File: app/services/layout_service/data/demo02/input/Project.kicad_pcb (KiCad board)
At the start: 2 copper layers, 48 x 48 mm, 57 parts, among them J1 M50-3500542, J2 NATTREY, T1 Thermistor_NTC, U1 AP7366-W5-7, U2 DRDC3105F-7, U3 TCM809RVNB713, U4 ATSAMD21G18A-MUT, U5 MX25L4006EM2I-12G, U6 LM35DZ/NOPB, U7 VEML6040A3OG, U8 ISM330DHCXTR, U9 BQ25101YFPR, X1 12 MHz, X2 32.768 kHz

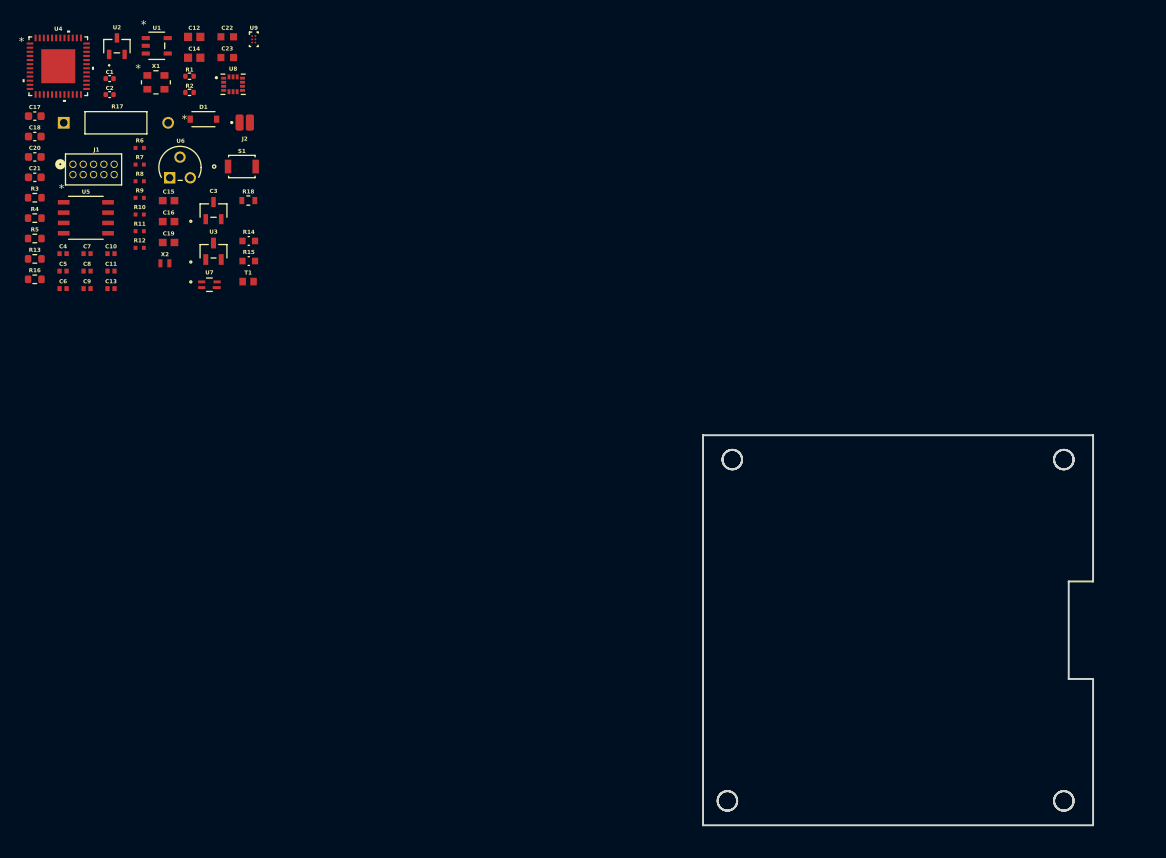
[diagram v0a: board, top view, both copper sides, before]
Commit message: 流程适配-反写网表-v2
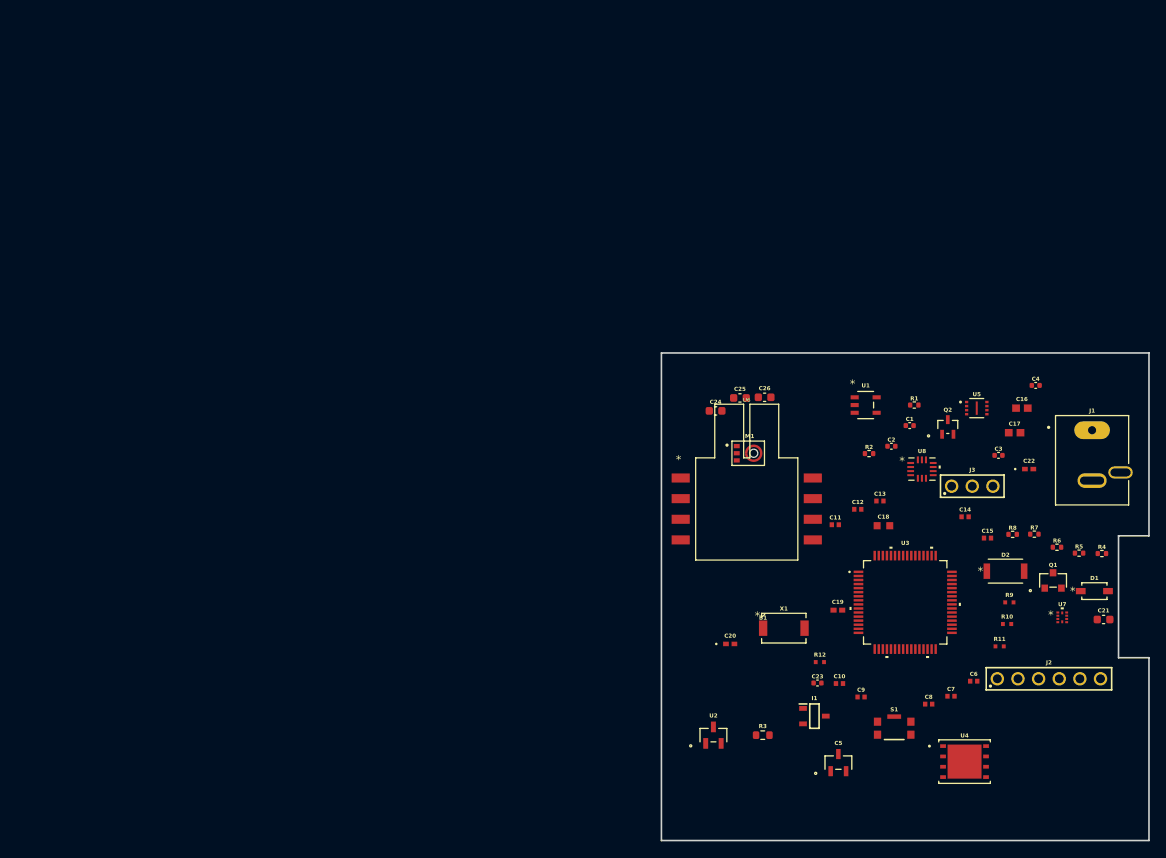
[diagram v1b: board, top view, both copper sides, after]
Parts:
- removed R13: 75R, LM35DZNOPB:R_0603_1608Metric
- removed R14, R15: 2.2K, VEML6040A3OG:RC0603N_YAG
- removed R16: 10k, ISM330DHCXTR:R_0603_1608Metric
- removed R17: 6K, BQ25101YFPR:CMF55_VIS
- removed R18: 1.35K, BQ25101YFPR:RES_RN73R_1J_KOA
- removed T1: Thermistor_NTC, BQ25101YFPR:TRES_NCP18XH103F03RB_MUR
- removed U9: BQ25101YFPR, BQ25101YFPR:YFP0006AFAV
- removed X2: 32.768 kHz, ATSAMD21G18A-MUT:ABS05_32_768KHZ_T
- added B1: Battery_CR1225, Battery_CR1225, F.Cu at (137.5, 109.2)
- added C24: C_0603_1608Metric, C_0603_1608Metric, F.Cu at (131.7, 77.1)
- added C25: C_0603_1608Metric, C_0603_1608Metric, F.Cu at (134.7, 75.5)
- added C26: C_0603_1608Metric, C_0603_1608Metric, F.Cu at (137.7, 75.5)
- added D2: SDO_CFP5_SOD128_NEX, SDO_CFP5_SOD128_NEX, F.Cu at (167.3, 96.8)
- added I1: SOT95P285X113-3N, SOT95P285X113-3N, F.Cu at (143.8, 114.7)
- added J3: 61300311121, 61300311121, F.Cu at (163.3, 86.4)
- added M1: MIC_ICS-40720, MIC_ICS-40720, F.Cu at (136.4, 82.3)
- added Q1: SOT-23_DIO, SOT-23_DIO, F.Cu at (173.2, 98.0)
- added Q2: SOT-323_DIO, SOT-323_DIO, F.Cu at (160.2, 79.1)
- C1, C2: value 1uF -> C_0402_1005Metric; footprint AP7366_W5_7:C_0402_1005Metric -> C_0402_1005Metric
- C10: value 1uF -> CAPC1005X55N; footprint ATSAMD21G18A-MUT:0402C -> 0402C
- C11, C6, C7: value 0.1uF -> CAPC1005X55N; footprint ATSAMD21G18A-MUT:0402C -> 0402C
- C12, C14: value 10uF -> CAPC1005X55N; footprint ATSAMD21G18A-MUT:0603C -> 0402C
- C13, C8: value 12 pF -> CAPC1005X55N; footprint ATSAMD21G18A-MUT:0402C -> 0402C
- C15: value 0.1uF -> CAPC1005X55N; footprint MX25L4006EM2I-12G:YAG_CC0603_YAG -> 0402C
- C16: value 0.01uF -> YAG_CC0603_YAG; footprint MX25L4006EM2I-12G:YAG_CC0603_YAG -> YAG_CC0603_YAG
- C17: value 0.01uF -> YAG_CC0603_YAG; footprint LM35DZNOPB:C_0603_1608Metric -> YAG_CC0603_YAG
- C18: value 1uF -> CAP_CL10A105KB8NNN_SAM; footprint LM35DZNOPB:C_0603_1608Metric -> CAP_CL10A105KB8NNN_SAM
- C19: value 0.1uF -> 0402_AVX; footprint VEML6040A3OG:YAG_CC0603_YAG -> 0402_AVX
- C20: value 0.1 uF -> CAP_0402_SAM; footprint ISM330DHCXTR:C_0603_1608Metric -> CAP_0402_SAM
- C21: value 0.1 uF -> C_0603_1608Metric; footprint ISM330DHCXTR:C_0603_1608Metric -> C_0603_1608Metric
- C22: value 1uF -> CAP_0402_SAM; footprint BQ25101YFPR:CAP_CL10A105KB8NNN_SAM -> CAP_0402_SAM
- C23: value 1uF -> C_0402_1005Metric; footprint BQ25101YFPR:CAP_CL10A105KB8NNN_SAM -> C_0402_1005Metric
- C3: value SM712-02HTG -> C_0402_1005Metric; footprint SM712-02HTG:SOT23-3_LTF -> C_0402_1005Metric
- C4: value 10 pF -> C_0402_1005Metric; footprint ATSAMD21G18A-MUT:0402C -> C_0402_1005Metric
- C5: value 0.1uF -> SOT23-3_LTF; footprint ATSAMD21G18A-MUT:0402C -> SOT23-3_LTF
- C9: value 10 pF -> CAPC1005X55N; footprint ATSAMD21G18A-MUT:0402C -> 0402C
- D1: value KDZVTR6.2B -> SOD-123_ONS; footprint DRDC3105F:DIO_KDZLVTF100_ROM -> SOD-123_ONS
- J1: value M50-3500542 -> CUI_PJ-044A; footprint ATSAMD21G18A-MUT:M50_3500542 -> CUI_PJ-044A
- J2: value NATTREY -> 61300611121; footprint BQ25101YFPR:SolderWirePad_1x02_SMD_1x2mm -> 61300611121
- R1: value 210K -> R_0402_1005Metric; footprint AP7366_W5_7:R_0402_1005Metric -> R_0402_1005Metric
- R10: value 1k -> RES_ERJ-2GEJ103X; footprint ATSAMD21G18A-MUT:0402R -> 0402R
- R11: value 330 -> RES_ERJ-2GEJ103X; footprint ATSAMD21G18A-MUT:0402R -> 0402R
- R12: value 10k -> RES_ERJ-2GEJ103X; footprint ATSAMD21G18A-MUT:0402R -> 0402R
- R2: value 40K -> R_0402_1005Metric; footprint AP7366_W5_7:R_0402_1005Metric -> R_0402_1005Metric
- R3: value 33K -> R_0603_1608Metric; footprint DRDC3105F:R_0603_1608Metric -> R_0603_1608Metric
- R4: value 1K -> R_0402_1005Metric; footprint DRDC3105F:R_0603_1608Metric -> R_0402_1005Metric
- R5: value 100K -> R_0402_1005Metric; footprint TCM809:R_0603_1608Metric -> R_0402_1005Metric
- R6, R7, R8: value 4.7k -> R_0402_1005Metric; footprint ATSAMD21G18A-MUT:0402R -> R_0402_1005Metric
- R9: value 4.7k -> RES_ERJ-2GEJ103X; footprint ATSAMD21G18A-MUT:0402R -> 0402R
- S1: value B3U-1000P -> SW_KMR221GLFS; footprint ATSAMD21G18A-MUT:B3U-1000P -> KMR221GLFS
- U1: value AP7366-W5-7 -> SOT25_DIO; footprint AP7366_W5_7:SOT25_DIO -> SOT25_DIO
- U2: value DRDC3105F-7 -> SOT-23_MC_MCH; footprint DRDC3105F:SOT23_MMBT2222A_NEX -> SOT-23_MC_MCH
- U3: value TCM809RVNB713 -> LQFP64-10x10mm; footprint TCM809:SOT-23_MC_MCH -> STM32F103RET6
- U4: value ATSAMD21G18A-MUT -> MR25H40CDC_EVS; footprint ATSAMD21G18A-MUT:QFN48_7X7MC_MCH -> MR25H40CDC_EVS
- U5: value MX25L4006EM2I-12G -> 8L_USON_2X3_ISI; footprint MX25L4006EM2I-12G:SOIC8_SOP8L_MAC -> 8L_USON_2X3_ISI
- U6: value LM35DZ/NOPB -> 1351-01_NXP; footprint LM35DZNOPB:Z03A -> 1351-01_NXP
- U7: value VEML6040A3OG -> MC3635_MEM; footprint VEML6040A3OG:LED_VEML6040A3OG_VIS -> MC3635_MEM
- U8: value ISM330DHCXTR -> BMX160_BOS; footprint ISM330DHCXTR:PQFN50P250X300X86-14N -> BMX160_BOS
- X1: value 12 MHz -> XTAL_NX5032GA-16.000M-STD-CSU-2_NDK; footprint ATSAMD21G18A-MUT:ABM8G_12_000MHZ_B4Y_T -> NX5032GA_16_000M_STD_CSU_2
- moved C21 142.3 mm to (179.4, 102.8)
- moved U4 140.6 mm to (162.3, 120.3)
- moved R4 137.7 mm to (179.2, 94.7)
- moved R5 134.2 mm to (176.4, 94.6)
- moved J1 130.6 mm to (178.0, 83.2)
- moved C17 126.7 mm to (168.5, 79.8)
- moved D1 124.1 mm to (178.3, 99.3)
- moved R6 123.1 mm to (173.7, 93.9)
- moved C6 122.0 mm to (163.4, 110.4)
- moved C4 120.8 mm to (171.1, 74.0)
- moved J2 120.3 mm to (172.7, 110.1)
- moved C7 119.5 mm to (160.6, 112.2)
- moved R7 119.1 mm to (170.9, 92.3)
- moved R10 118.0 mm to (167.5, 103.4)
- moved R9 118.0 mm to (167.8, 100.7)
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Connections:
- C1 pad 1: VOUT1 -> (no net)
- C1 pad 2: GND -> (no net)
- C10 pad 1: Net-(U4-VDDCORE) -> (no net)
- C10 pad 2: GND -> (no net)
- C11 pad 1: unconnected-(C11-Pad1) -> (no net)
- C11 pad 2: GND -> (no net)
- C12 pad 1: VOUT3 -> (no net)
- C12 pad 2: GND -> (no net)
- C13 pad 1: unconnected-(C13-Pad1) -> (no net)
- C13 pad 2: GND -> (no net)
- C14 pad 1: VOUT3 -> (no net)
- C14 pad 2: GND -> (no net)
- C15 pad 1: VOUT3 -> (no net)
- C15 pad 2: GND -> (no net)
- C16 pad 1: VOUT3 -> (no net)
- C16 pad 2: GND -> (no net)
- C17 pad 1: VOUT3 -> (no net)
- C17 pad 2: GND -> (no net)
- C18 pad 1: KLT7 -> (no net)
- C18 pad 2: Net-(C18-Pad2) -> (no net)
- C19 pad 1: VDD -> (no net)
- C19 pad 2: GND -> (no net)
- C2 pad 1: VOUT2 -> (no net)
- C2 pad 2: GND -> (no net)
- C20 pad 1: VOUT3 -> (no net)
- C20 pad 2: GND -> (no net)
- C21 pad 1: VOUT3 -> (no net)
- C21 pad 2: GND -> (no net)
- C22 pad 1: VIN -> (no net)
- C22 pad 2: GND -> (no net)
- C23 pad 1: VOUT -> (no net)
- C23 pad 2: GND -> (no net)
- C3 pad 1: KLT5 -> (no net)
- C3 pad 2: KLT6 -> (no net)
- C4 pad 1: unconnected-(C4-Pad1) -> (no net)
- C4 pad 2: GND -> (no net)
- C5 pad 1: VOUT3 -> (no net)
- C5 pad 2: GND -> (no net)
- C6 pad 1: VOUT3 -> (no net)
- C6 pad 2: GND -> (no net)
- C7 pad 1: VOUT3 -> (no net)
- C7 pad 2: GND -> (no net)
- C8 pad 1: KLT7 -> (no net)
- C8 pad 2: GND -> (no net)
- C9 pad 1: unconnected-(C9-Pad1) -> (no net)
- C9 pad 2: GND -> (no net)
- D1 pad 1: GND -> (no net)
- D1 pad 2: VOUT3 -> (no net)
- J1 pad 1: VOUT3 -> (no net)
- J1 pad 2: unconnected-(J1-Pad2) -> (no net)
- J1 pad 3: GND -> (no net)
- J2 pad 1: VOUT -> (no net)
- J2 pad 2: GND -> (no net)
- R1 pad 1: VOUT2 -> (no net)
- R1 pad 2: Net-(U1-ADJ) -> (no net)
- R10 pad 1: unconnected-(J1-Pad4) -> (no net)
- R10 pad 2: VOUT3 -> (no net)
- R11 pad 1: unconnected-(C11-Pad1) -> (no net)
- R11 pad 2: Net-(R11-Pad2) -> (no net)
- R12 pad 1: unconnected-(C11-Pad1) -> (no net)
- R12 pad 2: VOUT3 -> (no net)
- R2 pad 1: Net-(U1-ADJ) -> (no net)
- R2 pad 2: GND -> (no net)
- R3 pad 1: Net-(D2-K) -> (no net)
- R3 pad 2: GND -> (no net)
- R4 pad 1: Net-(D2-K) -> (no net)
- R4 pad 2: VOUT1 -> (no net)
- R5 pad 1: Net-(U3-*RESET) -> (no net)
- R5 pad 2: GND -> (no net)
- R6 pad 1: I2C_SDA -> (no net)
- R6 pad 2: VOUT3 -> (no net)
- R7 pad 1: unconnected-(R7-Pad1) -> (no net)
- R7 pad 2: VOUT3 -> (no net)
- R8 pad 1: unconnected-(R8-Pad1) -> (no net)
- R8 pad 2: VOUT3 -> (no net)
- R9 pad 1: I2C_SCL -> (no net)
- R9 pad 2: VOUT3 -> (no net)
- S1 pad 1: GND -> (no net)
- S1 pad 2: Net-(R11-Pad2) -> (no net)
- U1 pad 1: VOUT1 -> (no net)
- U1 pad 2: GND -> (no net)
- U1 pad 3: VOUT1 -> (no net)
- U1 pad 4: Net-(U1-ADJ) -> (no net)
- U1 pad 5: VOUT2 -> (no net)
- U2 pad 1: Net-(D2-K) -> (no net)
- U2 pad 2: GND -> (no net)
- U2 pad 3: VOUT3 -> (no net)
- U3 pad 1: VDD -> (no net)
- U3 pad 2: GND -> (no net)
- U3 pad 3: Net-(U3-*RESET) -> (no net)
- U4 pad 1: KLT7 -> (no net)
- U4 pad 2: unconnected-(U4-PA01-Pad2) -> (no net)
- U4 pad 3: unconnected-(U4-PA02-Pad3) -> (no net)
- U4 pad 4: unconnected-(U4-PA03-Pad4) -> (no net)
- U4 pad 5: GND -> (no net)
- U4 pad 6: VOUT3 -> (no net)
- U4 pad 7: unconnected-(U4-PB08-Pad7) -> (no net)
- U4 pad 8: unconnected-(U4-PB09-Pad8) -> (no net)
- U4 pad 9: unconnected-(U4-PA04-Pad9) -> (no net)
- U5 pad 1: unconnected-(U5-CS#-Pad1) -> (no net)
- U5 pad 2: unconnected-(U5-SO/SIO1-Pad2) -> (no net)
- U5 pad 3: unconnected-(U5-WP#-Pad3) -> (no net)
- U5 pad 4: GND -> (no net)
- U5 pad 5: KLT2 -> (no net)
- U5 pad 6: KLT3 -> (no net)
- U5 pad 7: KLT4 -> (no net)
- U5 pad 8: VOUT3 -> (no net)
- U6 pad 1: VOUT3 -> (no net)
- U6 pad 2: Net-(U6-Vout) -> (no net)
- U6 pad 3: GND -> (no net)
- U7 pad 1: GND -> (no net)
- U7 pad 2: I2C_SDA -> (no net)
- U7 pad 3: I2C_SCL -> (no net)
- U7 pad 4: VDD -> (no net)
- U8 pad 1: VOUT3 -> (no net)
- U8 pad 10: unconnected-(U8-OCS_AUX-Pad10) -> (no net)
- U8 pad 11: VOUT3 -> (no net)
- U8 pad 12: VOUT3 -> (no net)
- U8 pad 13: I2C_SCL -> (no net)
- U8 pad 14: I2C_SDA -> (no net)
- U8 pad 2: VOUT3 -> (no net)
- U8 pad 3: VOUT3 -> (no net)
- U8 pad 4: KLT0 -> (no net)
- U8 pad 5: VOUT3 -> (no net)
- U8 pad 6: GND -> (no net)
- U8 pad 7: GND -> (no net)
- U8 pad 8: VOUT3 -> (no net)
- U8 pad 9: KLT1 -> (no net)
- X1 pad 1: unconnected-(C9-Pad1) -> (no net)
- X1 pad 2: GND -> (no net)
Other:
- board size 48 x 48 mm -> 60 x 60 mm
